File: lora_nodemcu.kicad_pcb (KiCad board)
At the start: 4 copper layers, 11 parts, among them U1 RFM95, U2 LM1117-3.3

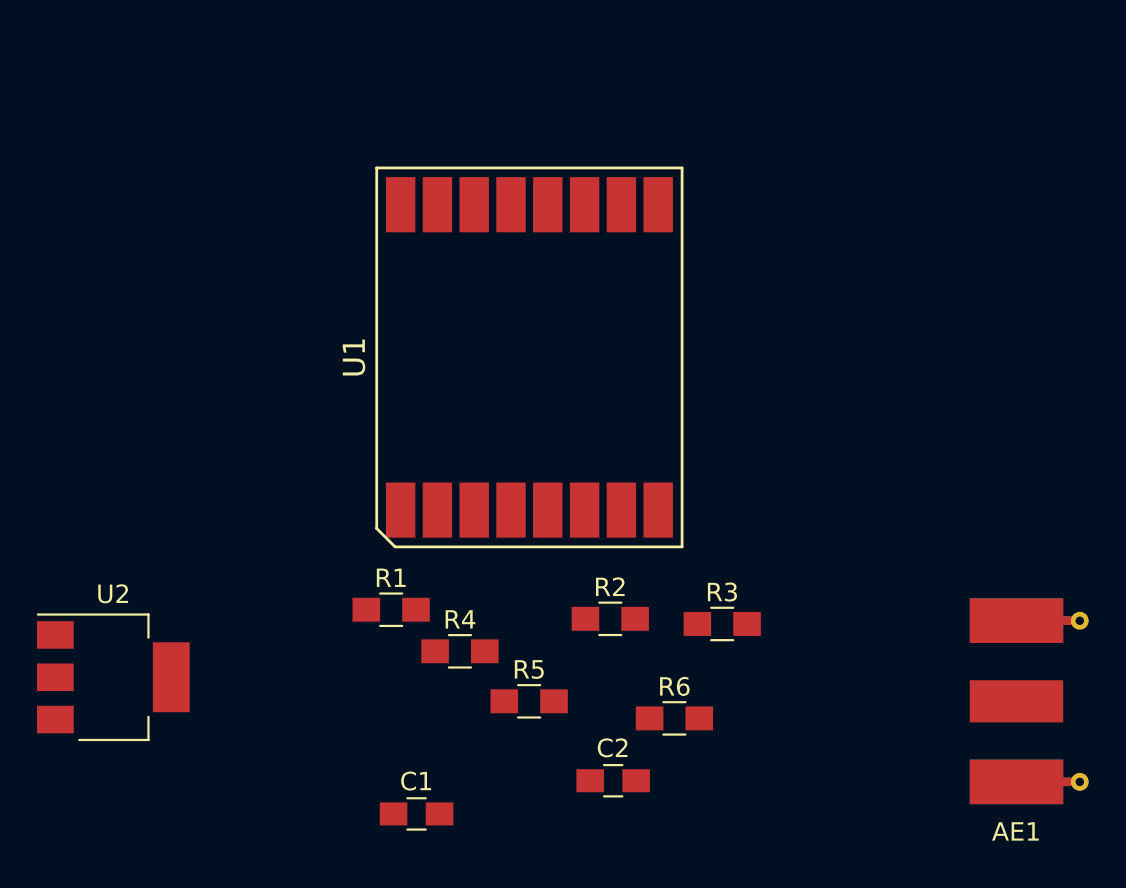
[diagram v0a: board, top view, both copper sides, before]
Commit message: Saving changes to circuit board prior to reworking yet again.
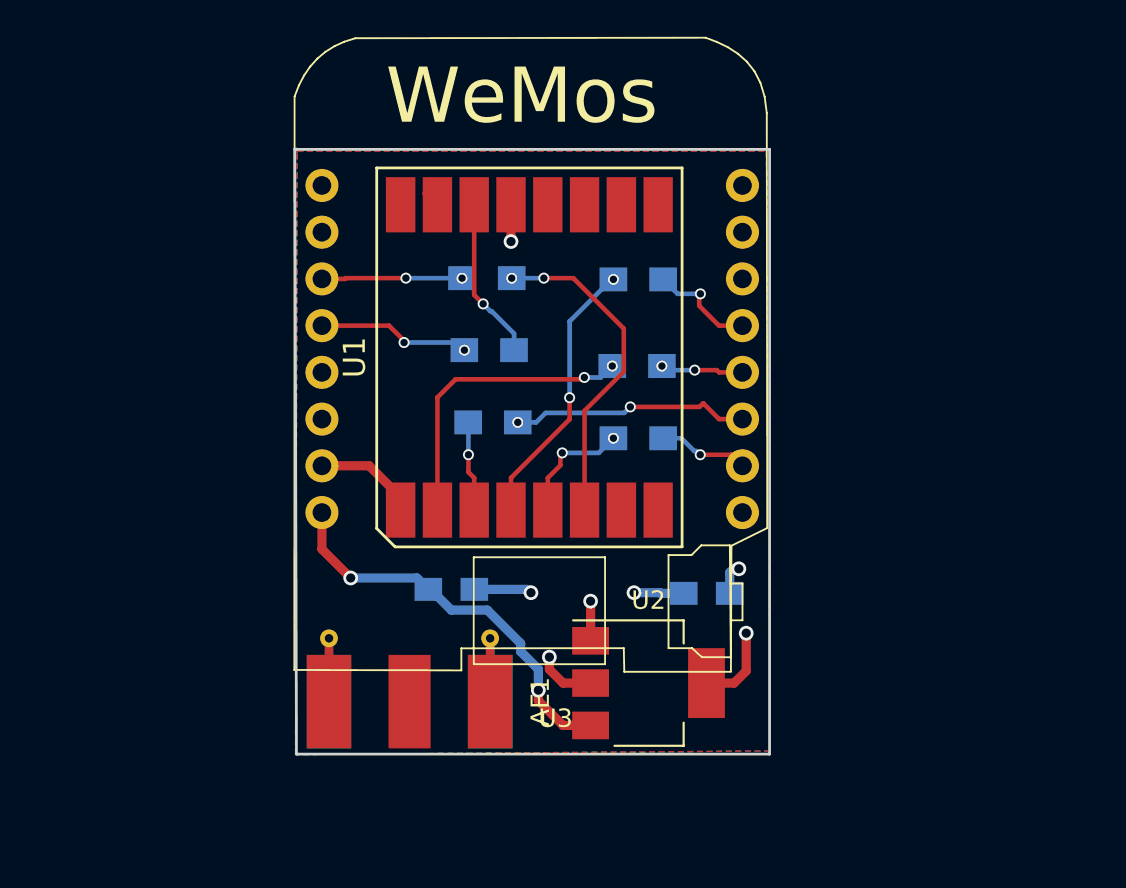
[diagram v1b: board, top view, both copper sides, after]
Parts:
- added U3: WeMos_mini, DisasterRadio:D1_mini_board, F.Cu at (148.7, 87.1)
- C1, C2, R1, R2, R3, R4, R5, R6: moved to B.Cu
- moved AE1 34.8 mm to (142.0, 103.3), turned to 90 degrees
- moved U2 29.1 mm to (155.0, 104.0)
- moved R4 22.4 mm to (154.4, 82.1), turned to 180 degrees
- moved R2 19.7 mm to (146.2, 82.0)
- moved R5 19.1 mm to (154.4, 86.8), turned to 180 degrees
- moved R6 18.9 mm to (146.5, 89.8), turned to 180 degrees
- moved R1 15.1 mm to (146.3, 85.9)
- moved C1 12.4 mm to (144.3, 98.9), turned to 180 degrees
- moved C2 11.4 mm to (158.2, 99.1)
- moved R3 11.1 mm to (154.4, 90.7), turned to 180 degrees
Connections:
- net Net-(AE1-Pad1) renamed /50Ohm
- U1 pad 10: GND -> Net-(U1-Pad10)
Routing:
- net +5V: track 0.00 -> 21.8 mm, vias 0 -> 2
- net Net-(R2-Pad2): track 0.00 -> 18.0 mm, vias 0 -> 2
- net Net-(R5-Pad2): track 0.00 -> 16.3 mm, vias 0 -> 2
- net Net-(R4-Pad2): track 0.00 -> 14.9 mm, vias 0 -> 2
- net GND: track 0.00 -> 13.7 mm, vias 0 -> 3
- net /MOSI: track 0.00 -> 13.0 mm, vias 0 -> 2
- net +3V3: track 0.00 -> 11.5 mm, vias 0 -> 4
- net Net-(R1-Pad2): track 0.00 -> 8.84 mm, vias 0 -> 1
- net Net-(R1-Pad1): track 0.00 -> 8.35 mm, vias 0 -> 2
- net Net-(R2-Pad1): track 0.00 -> 7.64 mm, vias 0 -> 2
- net Net-(R3-Pad2): track 0.00 -> 6.55 mm, vias 0 -> 2
- net /SCK: track 0.00 -> 5.83 mm, vias 0 -> 1
- net /SS: track 0.00 -> 4.93 mm, vias 0 -> 2
- net Net-(R6-Pad2): track 0.00 -> 4.91 mm, vias 0 -> 1
- net /MISO: track 0.00 -> 4.52 mm, vias 0 -> 2
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- added copper zone on In2.Cu, net +3V3
- added copper zone on B.Cu, net GND
- added copper zone on F.Cu, net GND
- added copper zone on In1.Cu, net GND
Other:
- board outline added: 25.8 x 32.9 mm
- net class power added: clearance 0.2, trace_width 0.5, via_dia 0.8, via_drill 0.5
